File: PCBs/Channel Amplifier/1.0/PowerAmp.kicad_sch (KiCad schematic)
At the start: 42 parts, among them J1 Conn_01x02_Male, J2 Conn_01x02_Male, J3 Conn_01x02_Male, J4 Conn_01x02_Male, J5 Conn_01x03_Male, J6 Conn_01x02_Male, J7 Conn_01x02_Male, J8 Conn_01x03_Male, J9 Conn_01x02_Male, U1 TMP100, U2 LM3886

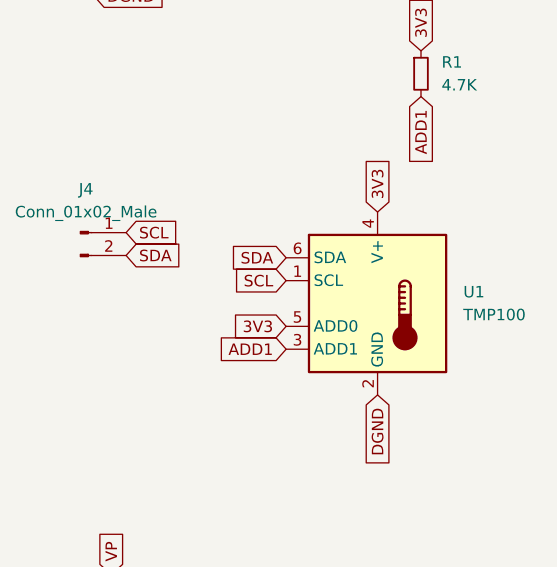
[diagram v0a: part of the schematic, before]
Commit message: KiCAD 7 updates
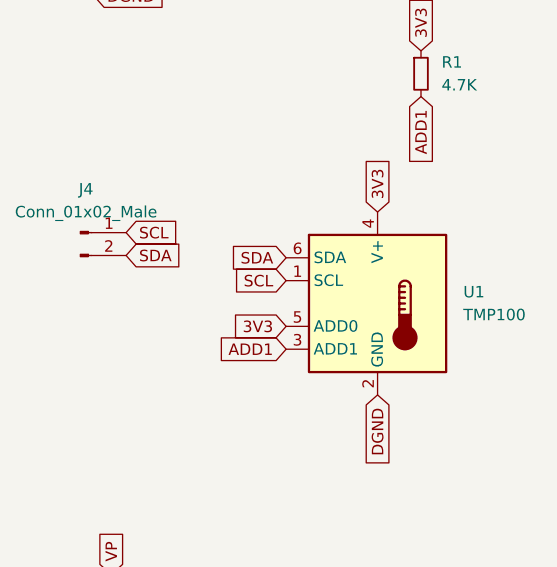
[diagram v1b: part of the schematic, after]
